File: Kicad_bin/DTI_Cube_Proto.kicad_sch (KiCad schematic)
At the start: 23 parts

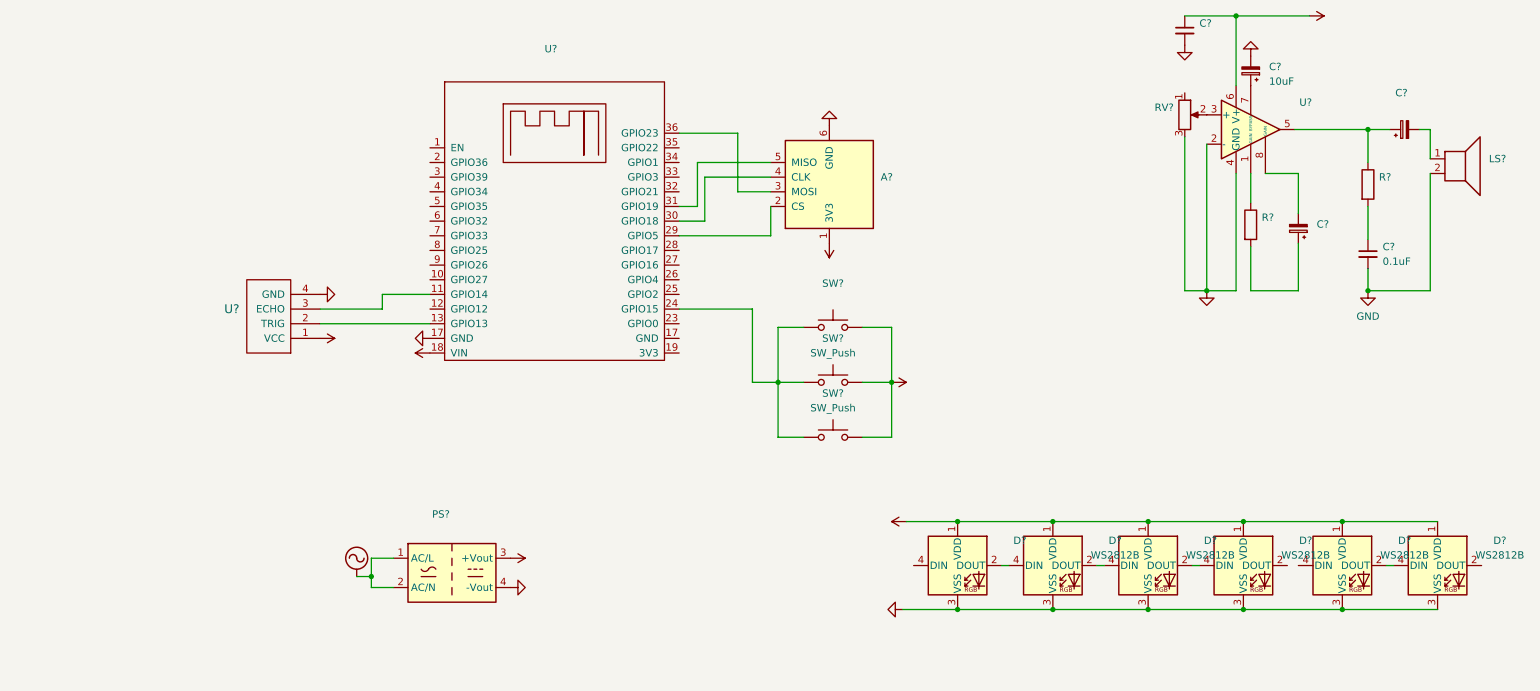
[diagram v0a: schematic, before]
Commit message: Schemy boi
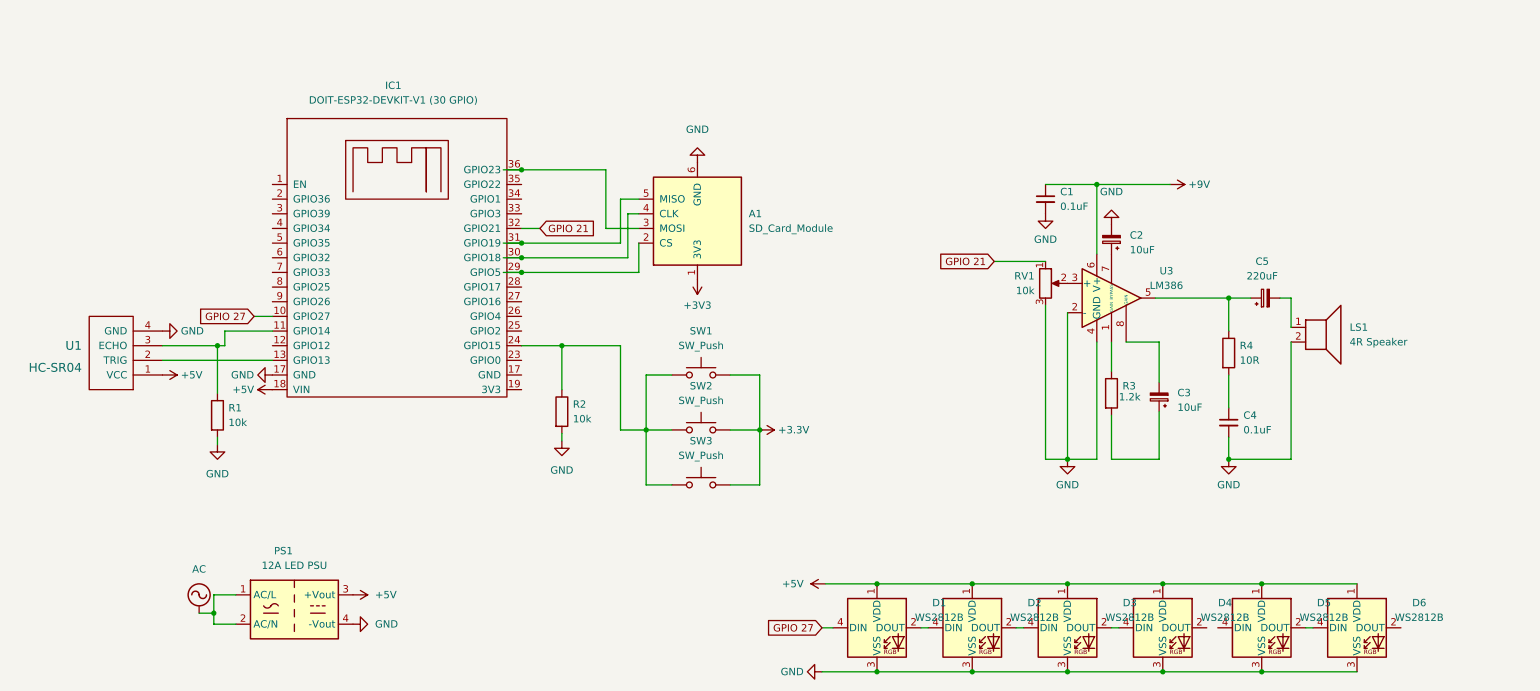
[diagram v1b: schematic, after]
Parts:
- added R1, R2: 10k, symbol Device:R
- A1: renamed from A?; value (none) -> SD_Card_Module; footprint (none) -> Charleslabs_Parts:SD_Card_Module
- C1: renamed from C?; value (none) -> 0.1uF
- C3: renamed from C?; value (none) -> 10uF
- C5: renamed from C?; value (none) -> 220uF
- D1: renamed from D?; value (none) -> WS2812B; footprint (none) -> LED_SMD:LED_WS2812B_PLCC4_5.0x5.0mm_P3.2mm
- IC1: renamed from U?; value (none) -> DOIT-ESP32-DEVKIT-V1 (30 GPIO)
- LS1: renamed from LS?; value (none) -> 4R Speaker
- PS1: renamed from PS?; value (none) -> 12A LED PSU; footprint (none) -> Converter_ACDC:Converter_ACDC_MeanWell_IRM-60-xx_THT
- R3: renamed from R?; value (none) -> 1.2k
- R4: renamed from R?; value (none) -> 10R
- RV1: renamed from RV?; value (none) -> 10k
- SW1: renamed from SW?; value (none) -> SW_Push
- U1: renamed from U?; value (none) -> HC-SR04
- U3: renamed from U?; value (none) -> LM386
- gave numbers to parts that had none: 9
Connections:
- net GND: now also R1.2, R2.2
- net GPIO 27: now reaches D1.4 (DIN)
- net GPIO 27: now also IC1.10 (GPIO27)
- net at IC1.24 (GPIO15), SW1.1, SW2.1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: now also R2.1
- net at IC1.11 (GPIO14), U1.3 (ECHO): now also R1.1
- net GPIO 21: now reaches IC1.32 (GPIO21)
- net GPIO 21: now also RV1.1
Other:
- company: (none) -> JVWCSY ☆
- title: (none) -> DTI Staircase Cube
- moved on the sheet: A1, C1, C2, C3, C4, C5, D1, D2, D3, D4, D5, D6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
